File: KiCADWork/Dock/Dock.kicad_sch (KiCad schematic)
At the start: 0 parts

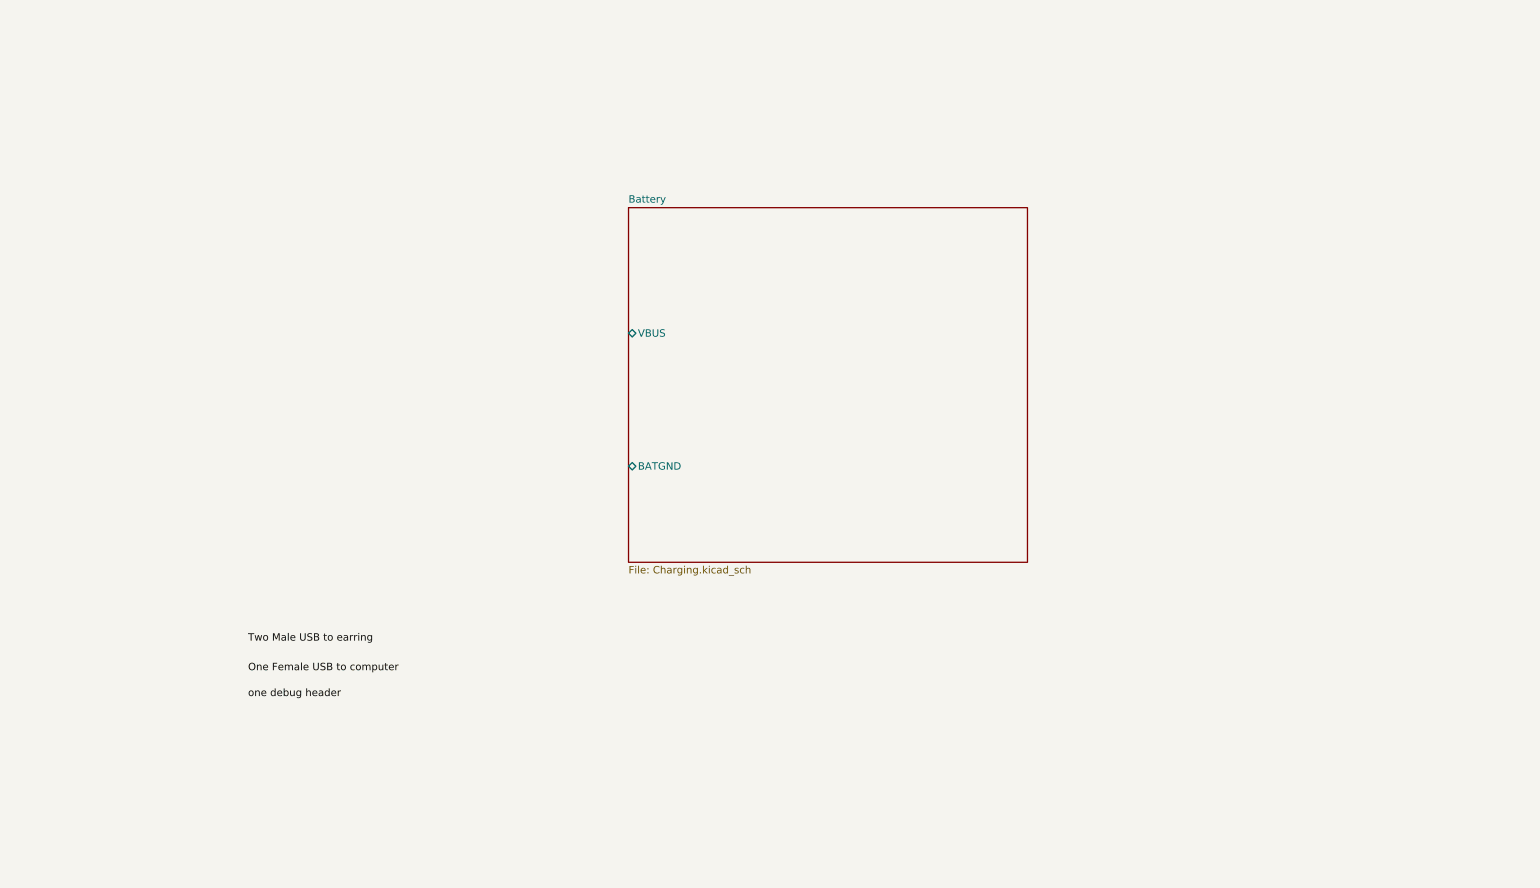
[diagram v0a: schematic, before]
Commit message: Dock Updates
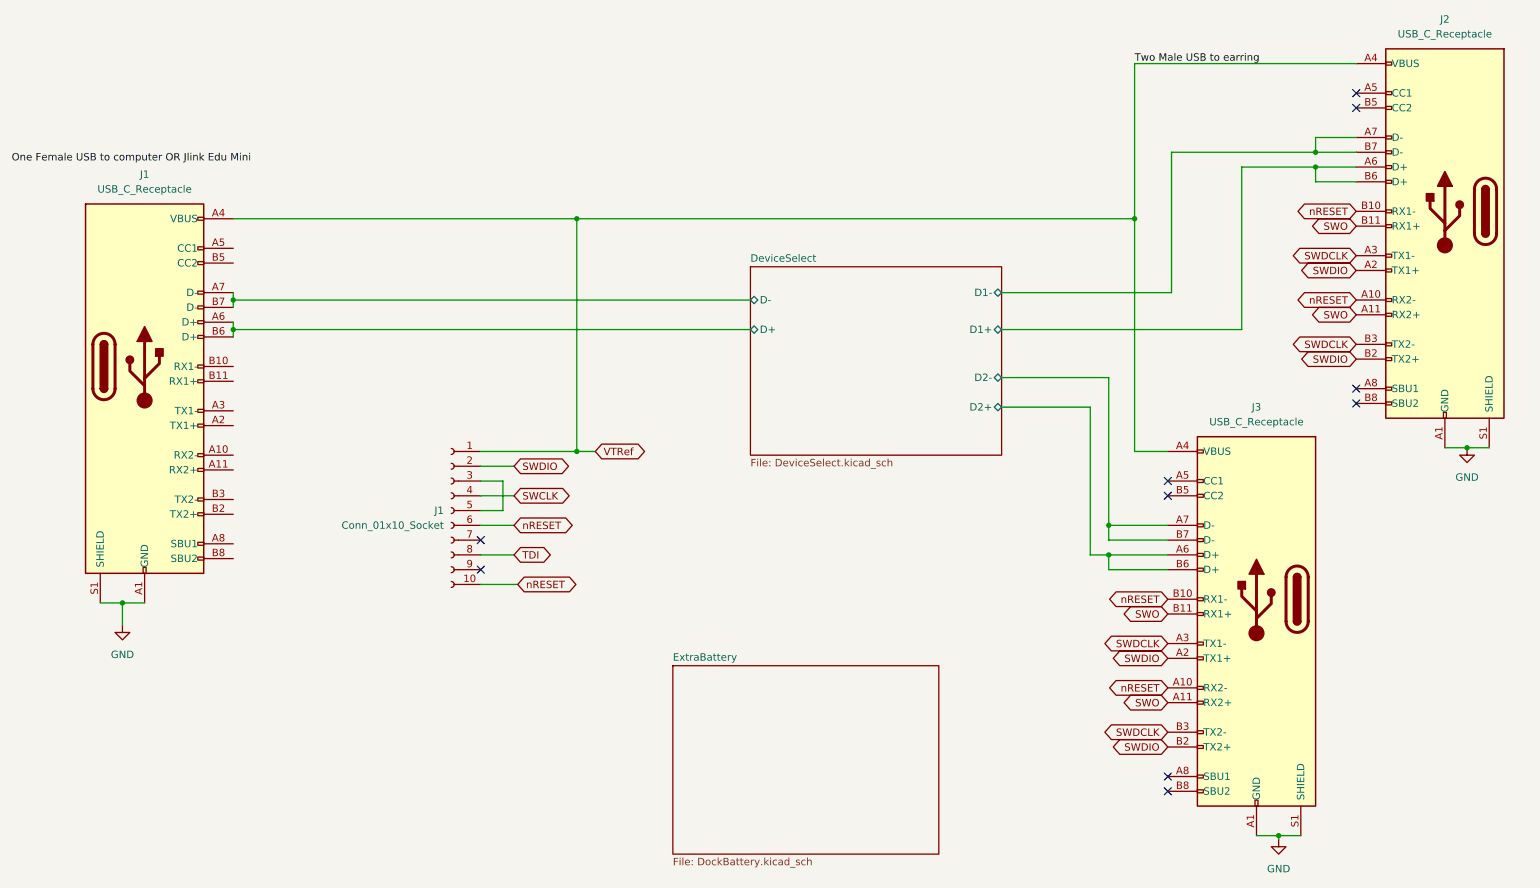
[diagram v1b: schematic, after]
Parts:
- added J1: Conn_01x10_Socket, easyeda2kicad:HDR-TH_10P-P1.27_X1321FR-2X05-C43D24, symbol Connector:Conn_01x10_Socket
- added J1: USB_C_Receptacle, easyeda2kicad:TYPE-C-SMD_C9900025773, symbol Connector:USB_C_Receptacle
- added J2, J3: USB_C_Receptacle, easyeda2kicad:USB-C-SMD_TYPEC-952-ACP24, symbol Connector:USB_C_Receptacle
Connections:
- new net: J1.3 (Pin_3), J1.5 (Pin_5)
- new net DeviceSelect/D+: J1.A6 (D+), J1.B6 (D+)
- new net DeviceSelect/D-: J1.A7 (D-), J1.B7 (D-)
- new net DeviceSelect/D1+: J2.A6 (D+), J2.B6 (D+)
- new net DeviceSelect/D1-: J2.A7 (D-), J2.B7 (D-)
- new net DeviceSelect/D2+: J3.A6 (D+), J3.B6 (D+)
- new net DeviceSelect/D2-: J3.A7 (D-), J3.B7 (D-)
- new net GND: J1.A1 (GND), J1.A12 (GND), J1.B1 (GND), J1.B12 (GND), J1.S1 (SHIELD), J2.A1 (GND), J2.A12 (GND), J2.B1 (GND), J2.B12 (GND), J2.S1 (SHIELD), J3.A1 (GND), J3.A12 (GND), J3.B1 (GND), J3.B12 (GND), J3.S1 (SHIELD)
- new net SWCLK: J1.4 (Pin_4)
- new net SWDCLK: J2.A3 (TX1-), J2.B3 (TX2-), J3.A3 (TX1-), J3.B3 (TX2-)
- new net SWDIO: J1.2 (Pin_2), J2.A2 (TX1+), J2.B2 (TX2+), J3.A2 (TX1+), J3.B2 (TX2+)
- new net SWO: J2.A11 (RX2+), J2.B11 (RX1+), J3.A11 (RX2+), J3.B11 (RX1+)
- new net TDI: J1.8 (Pin_8)
- new net VTRef: J1.1 (Pin_1), J1.A4 (VBUS), J1.A9 (VBUS), J1.B4 (VBUS), J1.B9 (VBUS), J2.A4 (VBUS), J2.A9 (VBUS), J2.B4 (VBUS), J2.B9 (VBUS), J3.A4 (VBUS), J3.A9 (VBUS), J3.B4 (VBUS), J3.B9 (VBUS)
- new net nRESET: J1.10 (Pin_10), J1.6 (Pin_6), J2.A10 (RX2-), J2.B10 (RX1-), J3.A10 (RX2-), J3.B10 (RX1-)
- no-connect marks 0 -> 10
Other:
- removed sheet Battery
- added sheet DeviceSelect (DeviceSelect.kicad_sch)
- added sheet ExtraBattery (DockBattery.kicad_sch)

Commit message: Dock Updates
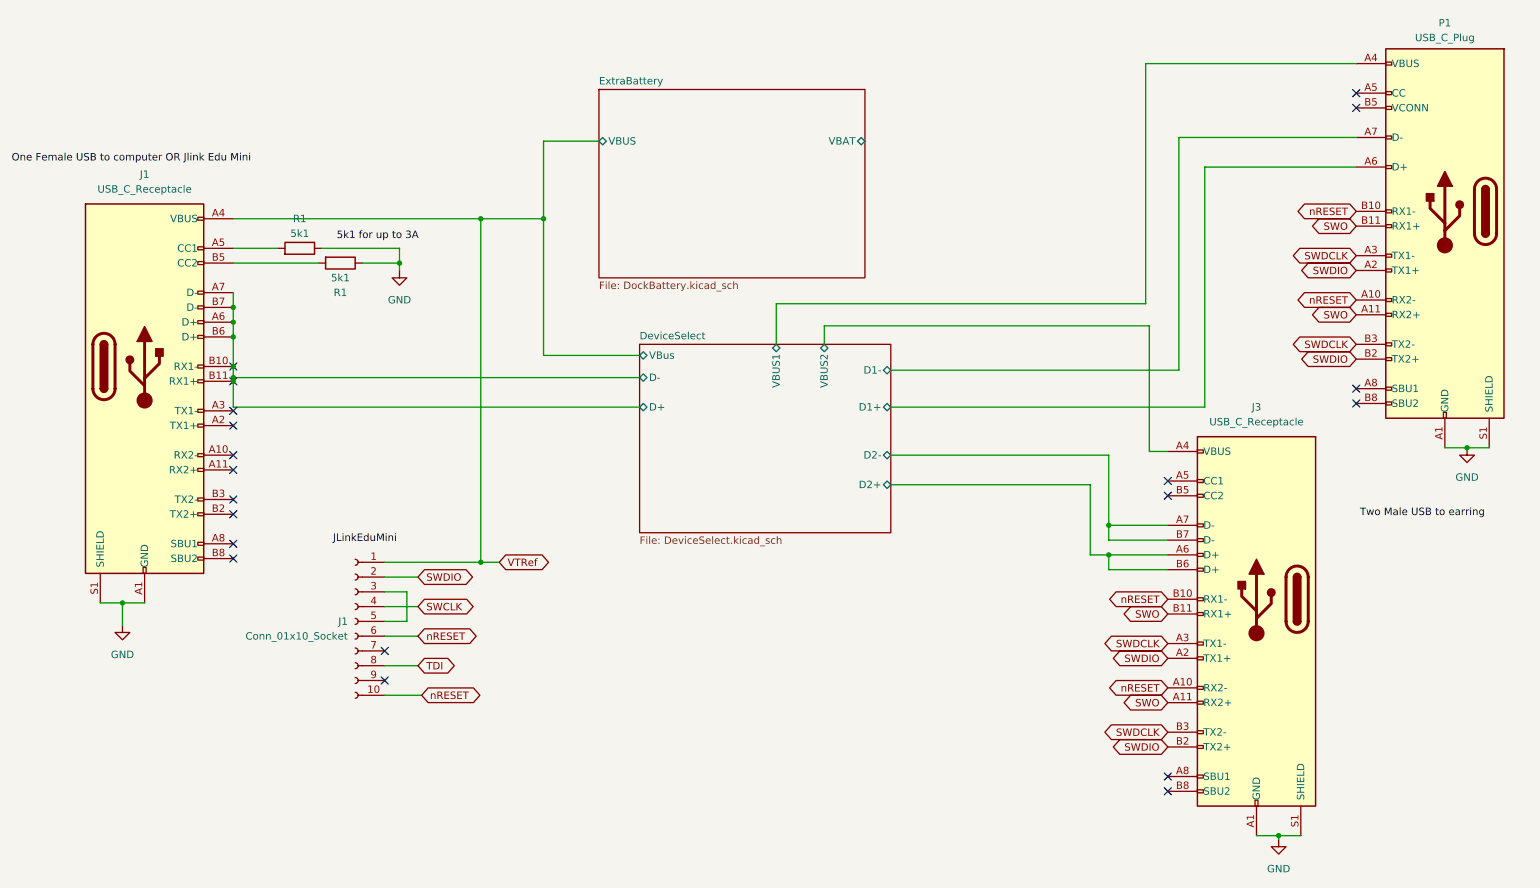
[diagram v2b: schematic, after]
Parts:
- removed J2: USB_C_Receptacle, easyeda2kicad:USB-C-SMD_TYPEC-952-ACP24, symbol Connector:USB_C_Receptacle
- added P1: USB_C_Plug, easyeda2kicad:USB-C-SMD_TYPEC-952-ACP24, symbol Connector:USB_C_Plug
- added R1 (x2): 5k1, Resistor_SMD:R_0402_1005Metric_Pad0.72x0.64mm_HandSolder, symbol Device:R
- J1: footprint easyeda2kicad:HDR-TH_10P-P1.27_X1321FR-2X05-C43D24 -> easyeda2kicad:HDR-TH_10P-P1.27-V-M-R2-C5-S1.27-1
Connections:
- net DeviceSelect/D- is gone; now on net DeviceSelect/D+: J1.A7 (D-), J1.B7 (D-)
- net DeviceSelect/D+: now also J1.B10 (RX1-), J1.B11 (RX1+)
- net DeviceSelect/D1+: now also P1.A6 (D+)
- net DeviceSelect/D1-: now also P1.A7 (D-)
- net GND: now also P1.A1 (GND), P1.A12 (GND), P1.B1 (GND), P1.B12 (GND), P1.S1 (SHIELD), R1.1, R1.1
- net SWDCLK: now also P1.A3 (TX1-), P1.B3 (TX2-)
- net SWDIO: now also P1.A2 (TX1+), P1.B2 (TX2+)
- net SWO: now also P1.A11 (RX2+), P1.B11 (RX1+)
- net VTRef: no longer J3.A4 (VBUS), J3.A9 (VBUS), J3.B4 (VBUS), J3.B9 (VBUS)
- net nRESET: now also P1.A10 (RX2-), P1.B10 (RX1-)
- net at J1.A5 (CC1): now also R1.2
- net at J1.B5 (CC2): now also R1.2
- new net DeviceSelect/VBUS1: P1.A4 (VBUS), P1.A9 (VBUS), P1.B4 (VBUS), P1.B9 (VBUS)
- new net DeviceSelect/VBUS2: J3.A4 (VBUS), J3.A9 (VBUS), J3.B4 (VBUS), J3.B9 (VBUS)
- no-connect marks 10 -> 20
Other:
- sheet DeviceSelect ports: added VBUS1, VBUS2, VBus; removed none
- sheet ExtraBattery ports: added VBAT, VBUS; removed none
- moved on the sheet: J1
